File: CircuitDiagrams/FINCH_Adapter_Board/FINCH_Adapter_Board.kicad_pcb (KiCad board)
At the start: 2 copper layers, 195 x 101.7 mm, 59 parts, among them J1 CONN_02X20, J2 CONN_02X25, J3 CONN_02X10, J4 CONN_01X07, J5 CONN_01X10, SW1 DIPS_04, U1 7417, U10 74LS163, U11 74LS163, U12 74LS163, U13 75107, U14 75110, U15 74LS08, U16 75107, U17 75107, U18 75110, U19 74LS163, U2 7417, U20 74LS163, U3 7416, U4 74LS138, U5 74LS109, U6 74LS00, U7 74LS125, U8 74LS04

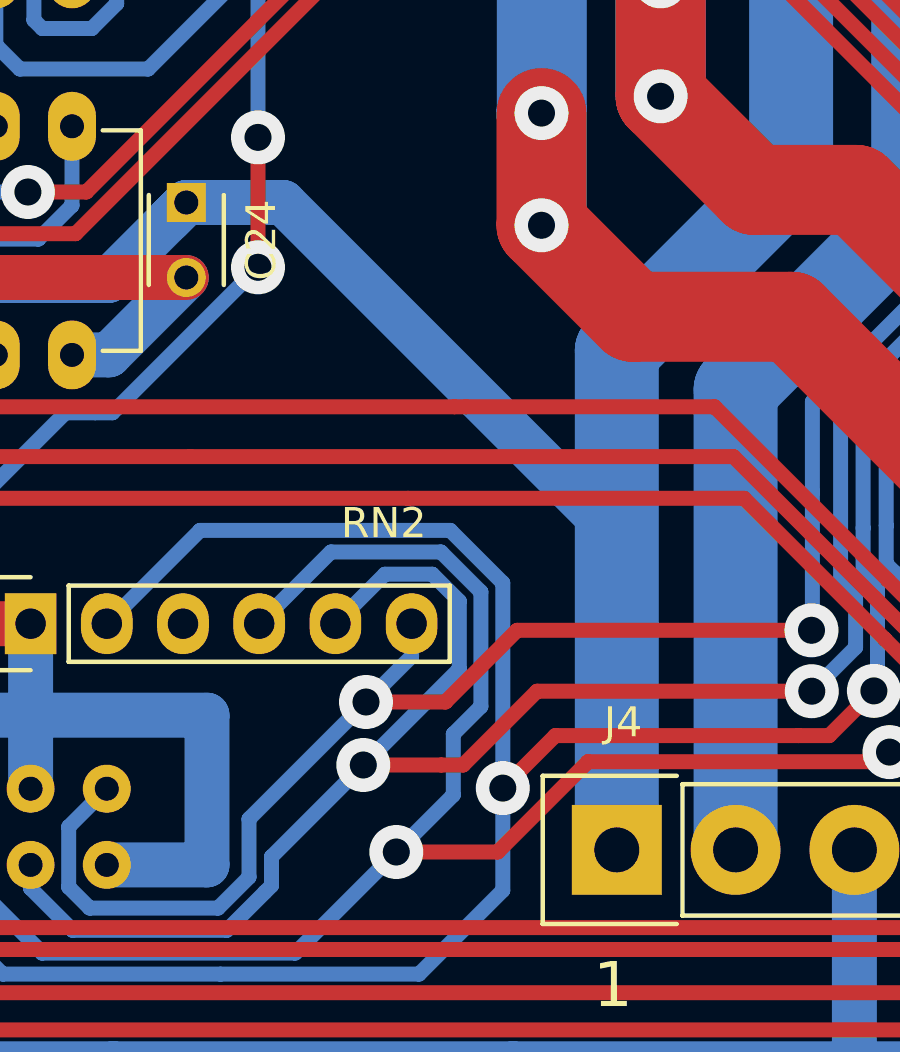
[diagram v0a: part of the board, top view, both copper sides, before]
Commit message: fix some stuff
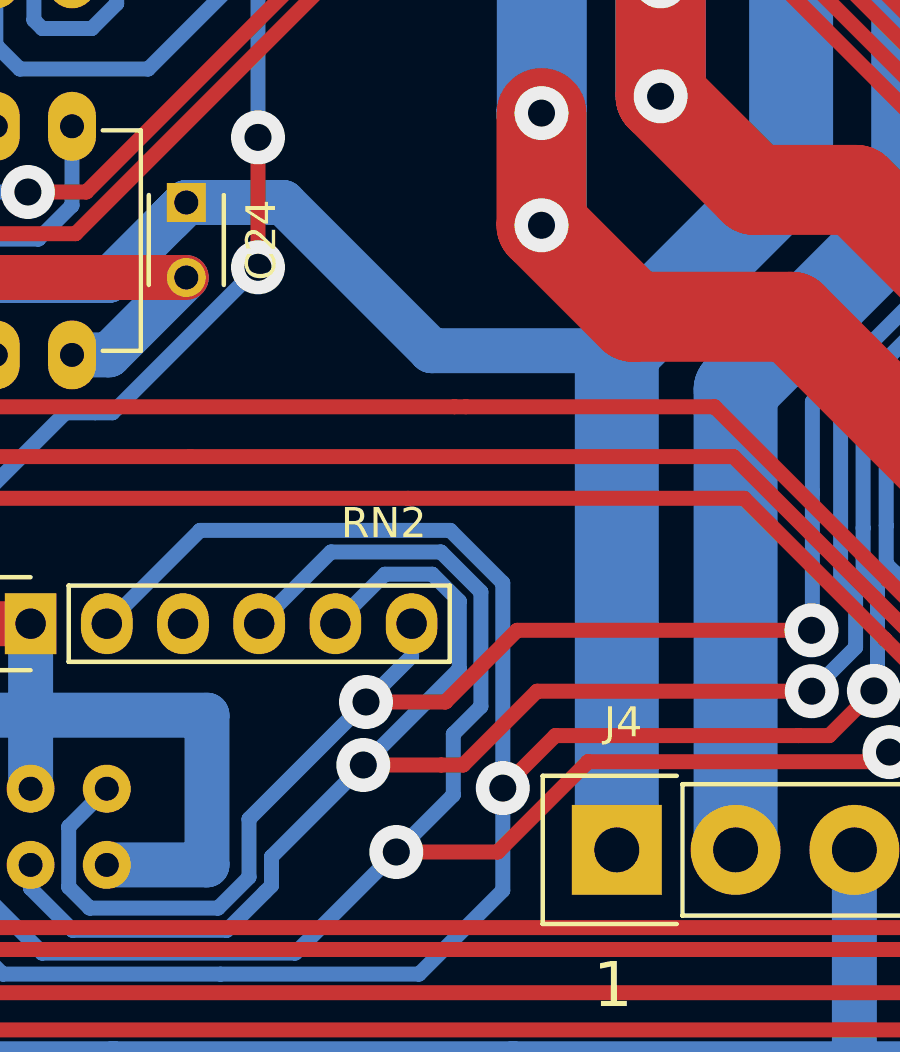
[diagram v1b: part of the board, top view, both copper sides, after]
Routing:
- net -5V: track 313.3 -> 300.3 mm
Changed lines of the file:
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@@
   (segment (start 53.57 135.7) (end 53.57 129.2) (width 1.5) (layer B.Cu) (net 2))
   (segment (start 146.44 135.7) (end 207.4 135.7) (width 1.5) (layer B.Cu) (net 2))
+  (segment (start 97.4 111.93) (end 91.22 111.93) (width 1.5) (layer B.Cu) (net 3))
+  (segment (start 91.22 111.93) (end 86.28 106.99) (width 1.5) (layer B.Cu) (net 3))
   (segment (start 85.61 106.99) (end 86.28 106.99) (width 1.5) (layer B.Cu) (net 3))
-  (segment (start 97.4 118.11) (end 97.4 128.57) (width 1.5) (layer B.Cu) (net 3))
-  (segment (start 86.28 106.99) (end 97.4 118.11) (width 1.5) (layer B.Cu) (net 3))
+  (segment (start 83.05 106.99) (end 85.61 106.99) (width 1.5) (layer B.Cu) (net 3))
   (segment (start 191.01 69.99) (end 195.78 69.99) (width 1.5) (layer F.Cu) (net 3))
   (segment (start 209.08 69.99) (end 210.64 69.99) (width 1.5) (layer F.Cu) (net 3))
@@
   (segment (start 71.62 108.09) (end 73.12 109.59) (width 1.5) (layer B.Cu) (net 3))
   (segment (start 82.47 107.57) (end 83.05 106.99) (width 1.5) (layer B.Cu) (net 3))
-  (segment (start 83.05 106.99) (end 85.61 106.99) (width 1.5) (layer B.Cu) (net 3))
   (segment (start 106.1 60.07) (end 103.21 62.96) (width 2.8) (layer B.Cu) (net 3))
   (segment (start 103.21 106.12) (end 97.4 111.93) (width 2.8) (layer B.Cu) (net 3))
